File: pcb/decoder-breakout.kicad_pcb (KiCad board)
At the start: 2 copper layers, 18 parts, among them J1 SM04B-SRSS-TB_LF__SN_, J2 SM04B-SRSS-TB_LF__SN_, J3 TBL009-254-08GY-2GY, Q1 BSS138, Q2 BSS138, U1 LS7866-S

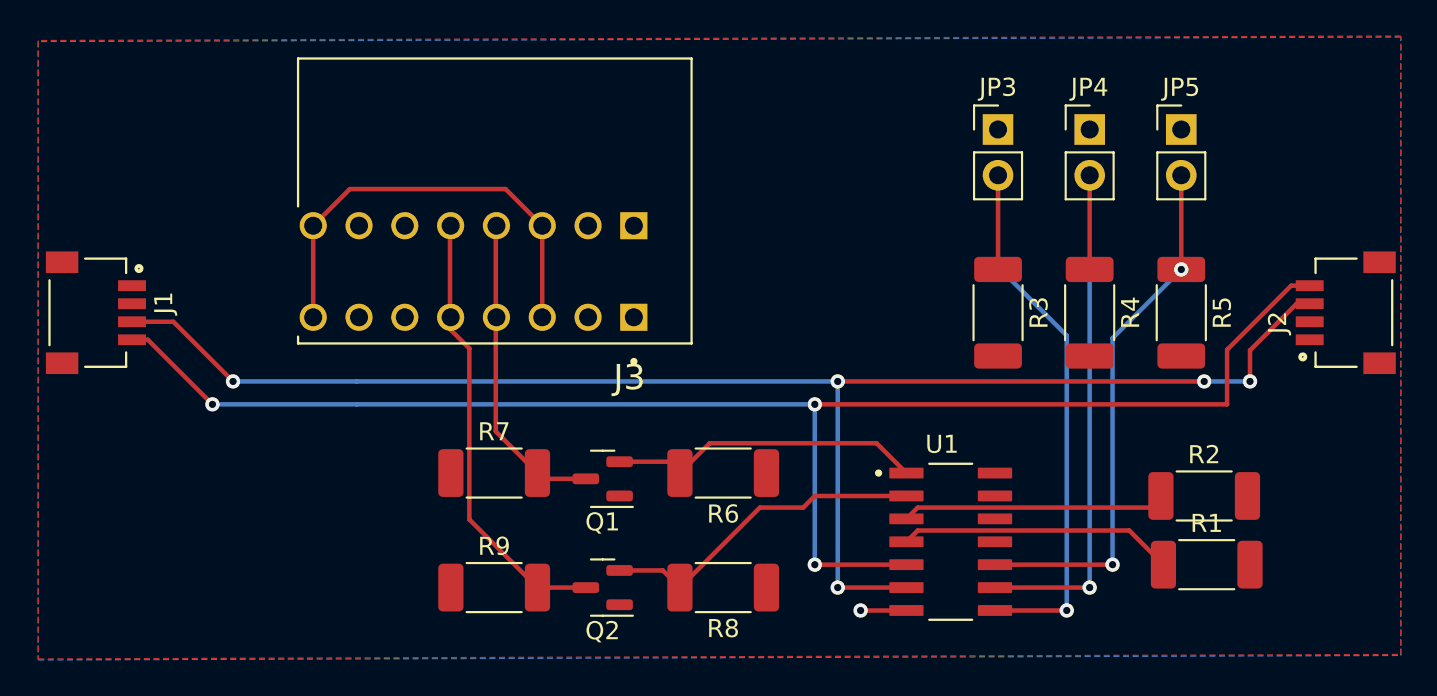
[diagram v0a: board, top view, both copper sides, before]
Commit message: working on copper fill
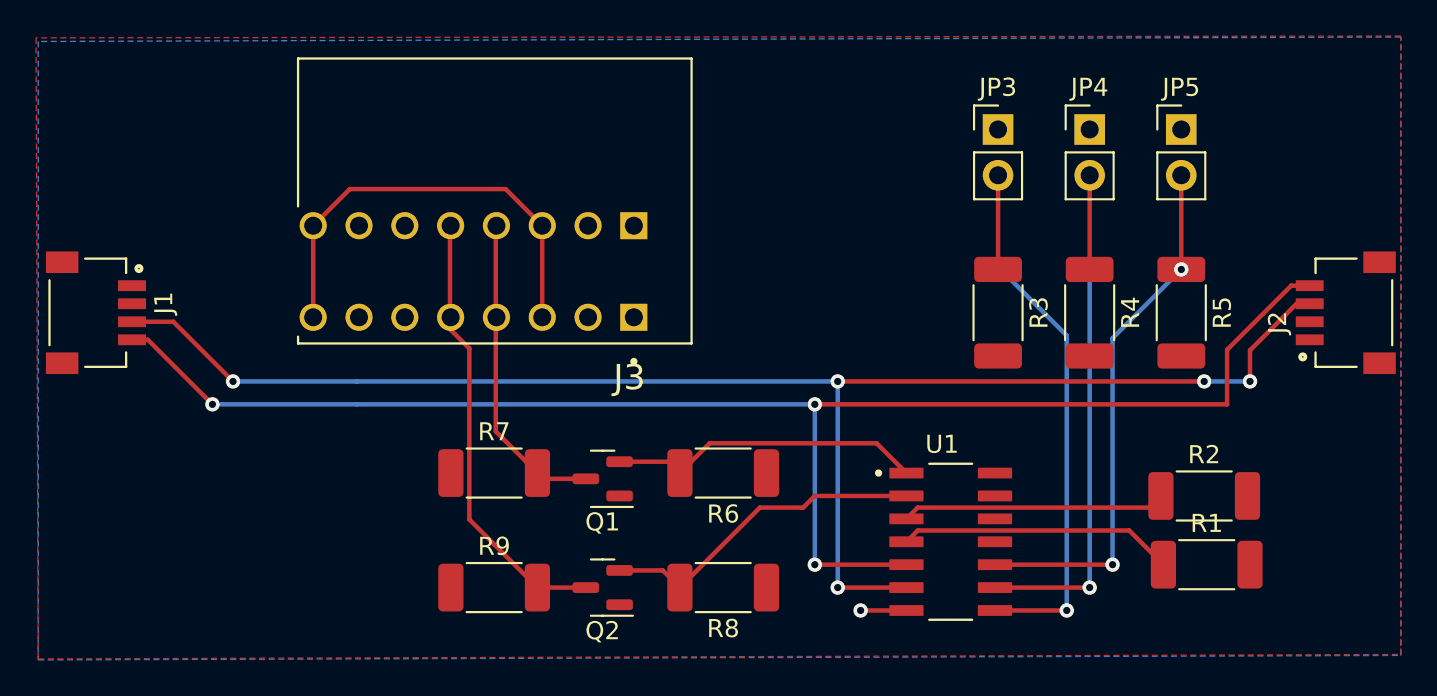
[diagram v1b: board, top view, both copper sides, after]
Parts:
- JP3, JP4, JP5: value Jumper_2_Bridged -> (none)
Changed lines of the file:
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@@
         (effects (font (size 1 1) (thickness 0.15)))
     )
-    (fp_text value "Jumper_2_Bridged" (at 0 4.87) (layer "F.Fab")
+    (fp_text value " " (at 0 4.87) (layer "F.Fab")
         (effects (font (size 1 1) (thickness 0.15)))
     )
@@
         (effects (font (size 1 1) (thickness 0.15)))
     )
-    (fp_text value "Jumper_2_Bridged" (at 0 4.87) (layer "F.Fab")
+    (fp_text value " " (at 0 4.87) (layer "F.Fab")
         (effects (font (size 1 1) (thickness 0.15)))
     )
@@
         (effects (font (size 1 1) (thickness 0.15)))
     )
-    (fp_text value "Jumper_2_Bridged" (at 0 4.87) (layer "F.Fab")
+    (fp_text value " " (at 0 4.87) (layer "F.Fab")
         (effects (font (size 1 1) (thickness 0.15)))
     )
@@
   (segment (start 140.97 105.41) (end 140.97 92.85) (width 0.25) (layer "B.Cu") (net 18))
   (zone (net 2) (net_name "VDD") (layer "F.Cu") (hatch edge 0.5)
-    (priority 1)
     (connect_pads (clearance 0.5))
     (min_thickness 0.25) (filled_areas_thickness no)
@@
     (polygon
       (pts
-        (xy 81.4 76.35)
+        (xy 81.28 76.2)
         (xy 81.4 110.64)
         (xy 156.95 110.39)
@@
     (connect_pads (clearance 0.5))
     (min_thickness 0.25) (filled_areas_thickness no)
-    (fill (thermal_gap 0.5) (thermal_bridge_width 0.5))
+    (fill yes (thermal_gap 0.5) (thermal_bridge_width 0.5))
     (polygon
       (pts
